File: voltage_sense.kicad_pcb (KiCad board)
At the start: 6 copper layers, 48 x 34 mm, 58 parts, among them IC1 DAC101C081CIMK_NOPB, J1 Conn_Coaxial, J2 Conn_01x04, J4 HDMI_A, J5 Conn_Coaxial, U1 OPA188xxDBV, U2 ADA4000-1, U3 OPA188xxDBV, U4 MCP4017T-103E_LT, U5 OPA1641, U6 24AA025UID, U9 LP2981A-33DBVT

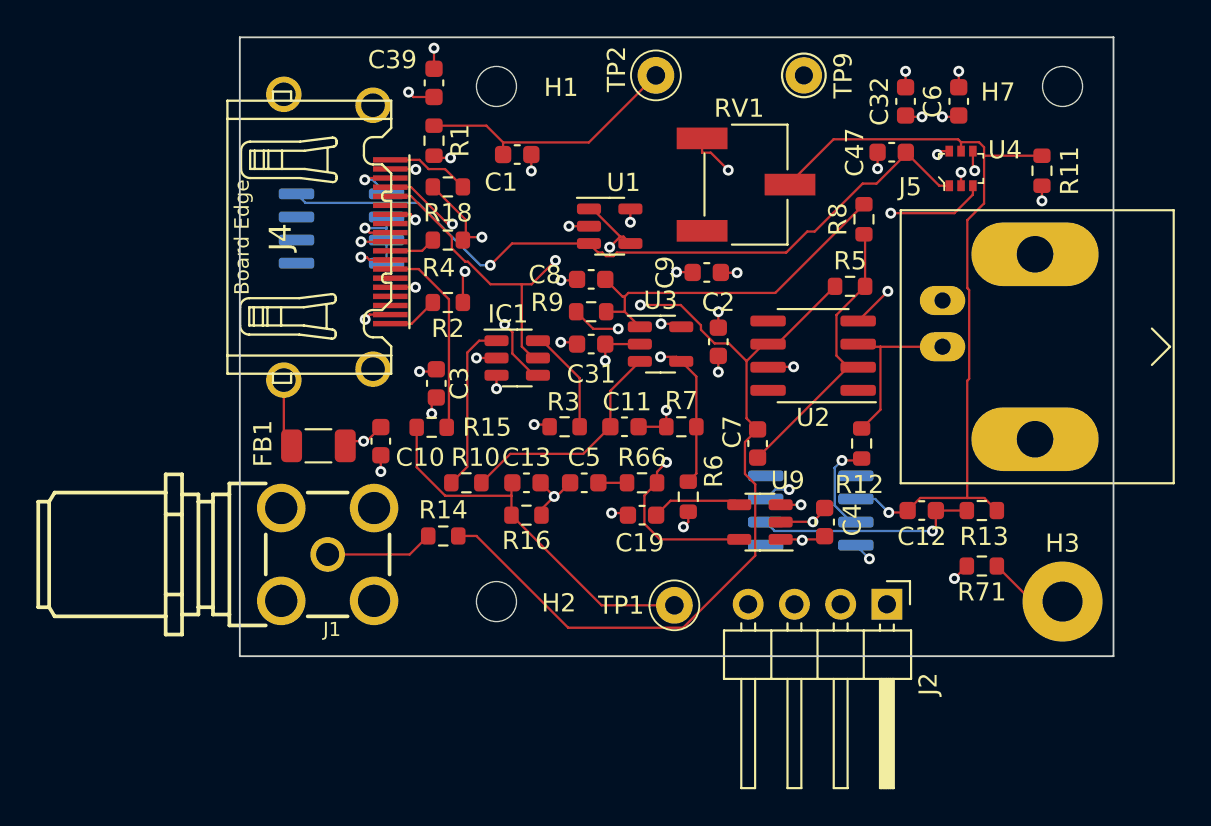
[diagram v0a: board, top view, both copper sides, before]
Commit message: Add files via upload
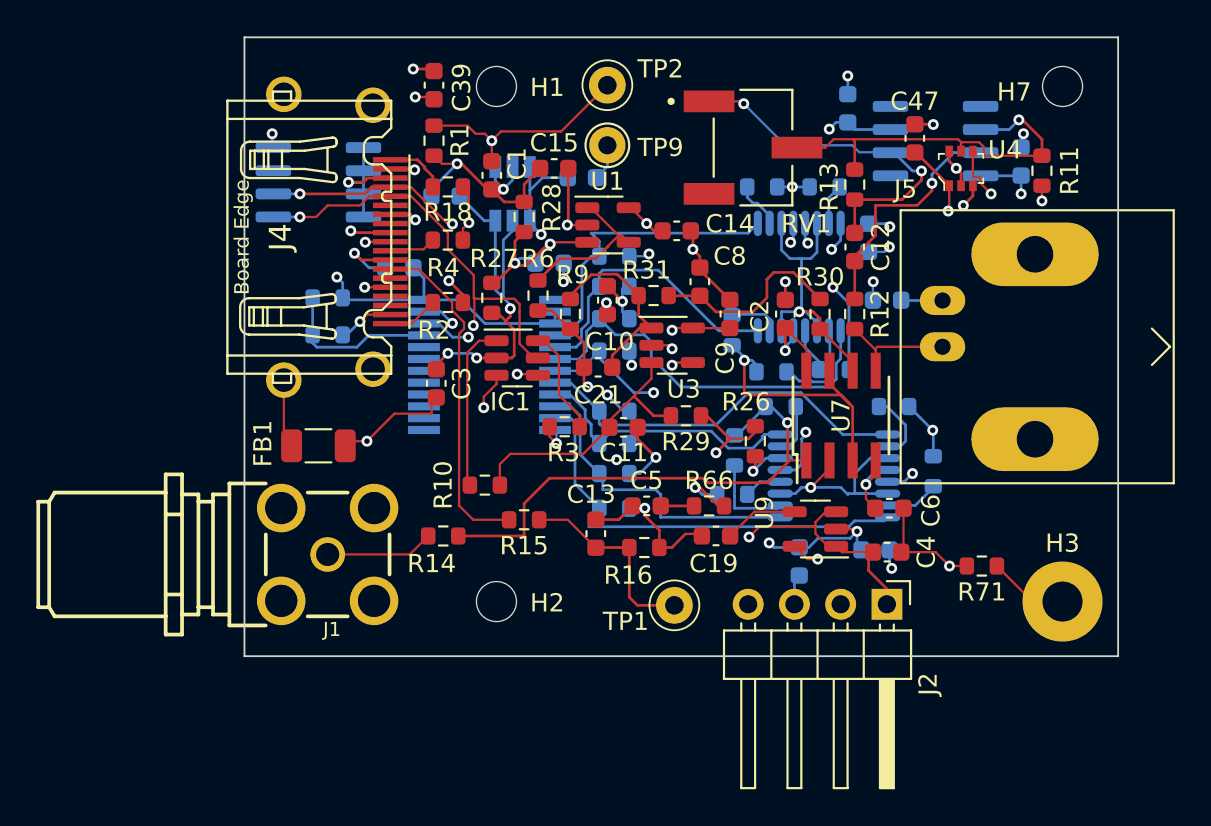
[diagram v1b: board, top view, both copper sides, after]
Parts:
- removed R7: 27.4k, Resistor_SMD:R_0603_1608Metric
- added C14: 0.1u, Capacitor_SMD:C_0603_1608Metric, F.Cu at (24.0, -23.4)
- added C15: 0.1u, Capacitor_SMD:C_0603_1608Metric, F.Cu at (17.3, -26.8)
- added C16: 0.1u, Capacitor_SMD:C_0603_1608Metric, B.Cu at (35.6, -19.6)
- added C17: 0.1u, Capacitor_SMD:C_0603_1608Metric, B.Cu at (34.5, -23.0)
- added C18: 0.1u, Capacitor_SMD:C_0603_1608Metric, B.Cu at (30.7, -5.21)
- added C20: 0.1u, Capacitor_SMD:C_0603_1608Metric, B.Cu at (34.9, -5.84)
- added C21: 10p, Capacitor_SMD:C_0603_1608Metric, F.Cu at (19.7, -15.9)
- added C22: 0.1u, Capacitor_SMD:C_0603_1608Metric, B.Cu at (18.8, -26.3)
- added C23: 1u, Capacitor_SMD:C_0603_1608Metric, B.Cu at (11.3, -25.3)
- added C24: 1u, Capacitor_SMD:C_0603_1608Metric, B.Cu at (17.0, -21.6)
- added R17: 100k, Resistor_SMD:R_0603_1608Metric, B.Cu at (20.6, -22.0)
- added R19: 100k, Resistor_SMD:R_0603_1608Metric, B.Cu at (20.6, -13.5)
- added R20: 100k, Resistor_SMD:R_0603_1608Metric, B.Cu at (20.6, -20.3)
- added R21: 100k, Resistor_SMD:R_0603_1608Metric, B.Cu at (20.6, -11.7)
- added R22: 100k, Resistor_SMD:R_0603_1608Metric, B.Cu at (20.6, -18.5)
- added R23: 100k, Resistor_SMD:R_0603_1608Metric, B.Cu at (20.6, -10.0)
- added R24: 100k, Resistor_SMD:R_0603_1608Metric, B.Cu at (20.6, -16.8)
- added R25: 100k, Resistor_SMD:R_0603_1608Metric, B.Cu at (20.6, -8.13)
- added R26: 3.01k, Resistor_SMD:R_0603_1608Metric, F.Cu at (28.3, -11.8)
- added R27: 10k, Resistor_SMD:R_0603_1608Metric, F.Cu at (13.8, -19.7)
- added R28: 10k, Resistor_SMD:R_0603_1608Metric, F.Cu at (15.6, -24.1)
- added R29: 4.99k, Resistor_SMD:R_0603_1608Metric, F.Cu at (24.5, -13.2)
- added R30: 3.01k, Resistor_SMD:R_0603_1608Metric, F.Cu at (31.9, -18.8)
- added R31: 49.9, Resistor_SMD:R_0603_1608Metric, F.Cu at (22.7, -19.8)
- added R32: DNI, Resistor_SMD:R_0603_1608Metric, B.Cu at (32.6, -15.7)
- added R33: 226k, Resistor_SMD:R_0603_1608Metric, B.Cu at (28.7, -25.8)
- added R34: 348k, Resistor_SMD:R_0603_1608Metric, B.Cu at (27.1, -17.9)
- added R35: 470k, Resistor_SMD:R_0603_1608Metric, B.Cu at (29.2, -15.6)
- added R36: 604k, Resistor_SMD:R_0603_1608Metric, B.Cu at (32.1, -25.8)
- added R38: DNI, Resistor_SMD:R_0603_1608Metric, B.Cu at (27.1, -8.89)
- added R39: 226k, Resistor_SMD:R_0603_1608Metric, B.Cu at (35.9, -13.7)
- added R40: 348k, Resistor_SMD:R_0603_1608Metric, B.Cu at (29.7, -13.7)
- added R41: 470k, Resistor_SMD:R_0603_1608Metric, B.Cu at (27.2, -11.3)
- added R42: 604k, Resistor_SMD:R_0603_1608Metric, B.Cu at (38.1, -10.2)
- added U10: TMUX6111PWR, covg-kicad:PW0016A_N, B.Cu at (32.6, -9.91)
- added U11: REF3440TIDBVR, covg-kicad:REF3440, B.Cu at (15.0, -25.4)
- added U7: ADA4000-2ARZ-R7, covg-kicad:R_8_ADI, F.Cu at (33.0, -13.2)
- added U8: TMUX6111PWR, covg-kicad:PW0016A_N, B.Cu at (30.7, -20.8)
- C11: value 0.1u -> 1u
- C31, C32: moved to B.Cu
- C7: value 4p -> 0.1u; moved to B.Cu
- C8: value 0.1u -> 1n
- J2: value Conn_01x04 -> DNI
- R10: value 27.4k -> 49.9k
- R12: value DNI -> 0
- R5: value 60.4k -> 100k; moved to B.Cu
- R6: value 33.2k -> 49.9k
- R8: value 3.01k -> DNI; moved to B.Cu
- R9: value 10k -> 4.99k
- RV1: footprint Potentiometer_SMD:Potentiometer_Bourns_3269W_Vertical -> covg-kicad:TRIM_3269W-1-103GLF
- U2: value ADA4000-1 -> TCA9555DBR; footprint Package_SO:SOIC-8_3.9x4.9mm_P1.27mm -> Package_SO:SSOP-24_5.3x8.2mm_P0.65mm; moved to B.Cu
- moved R8 30.1 mm to (4.83, -17.7), turned to 0 degrees
- moved R5 28.7 mm to (4.83, -19.7)
- moved C31 25.7 mm to (42.9, -27.2), turned to -90 degrees
- moved C6 22.7 mm to (35.7, -8.13), turned to 0 degrees
- moved C7 21.9 mm to (8.76, -21.3), turned to 0 degrees
- moved U5 21.4 mm to (38.2, -28.3)
- moved R13 19.2 mm to (33.8, -25.9), turned to 90 degrees
- moved U2 17.8 mm to (13.7, -16.0)
- moved C12 14.9 mm to (33.8, -22.5), turned to -90 degrees
- moved C10 14.7 mm to (20.2, -19.6)
- moved R6 13.8 mm to (16.4, -19.8), turned to 90 degrees
- moved TP9 11.5 mm to (20.2, -28.1)
- moved R15 7.18 mm to (15.6, -7.49), turned to 180 degrees
- moved R12 7.12 mm to (33.8, -18.8), turned to -90 degrees
- moved R16 6.72 mm to (22.2, -5.97)
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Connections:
- net 3V3_BUF renamed /vsense/2V_BUF
- C3 pad 2: +5V -> +4V
- C7 pad 1: Net-(C7-Pad1) -> GND
- C7 pad 2: Net-(C7-Pad2) -> +3V3
- IC1 pad 2: +5V -> +4V
- IC1 pad 4: /vsense/SDA -> SDA
- IC1 pad 5: /vsense/SCL -> SCL
- J4 pad 15: /vsense/SCL -> SCL
- J4 pad 16: /vsense/SDA -> SDA
- R11 pad 2: Net-(C12-Pad2) -> Net-(R11-Pad2)
- R12 pad 1: Net-(R12-Pad1) -> Net-(C12-Pad2)
- R13 pad 2: Net-(C12-Pad2) -> Net-(R11-Pad2)
- R14 pad 2: Net-(C7-Pad2) -> /vsense/gain_adjust_2/OUT
- R18 pad 1: /vsense/AMP_OUT -> /vsense/STG1_OUT
- R18 pad 2: Net-(C7-Pad2) -> /vsense/AMP_OUT
- R4 pad 1: /vsense/CAL_ADC -> /vsense/STG1_OUT
- R4 pad 2: Net-(C7-Pad2) -> /vsense/CAL_ADC
- R5 pad 1: Net-(C7-Pad1) -> +3V3
- R5 pad 2: Net-(C7-Pad2) -> Net-(R5-Pad2)
- R8 pad 1: Net-(C7-Pad1) -> Net-(R5-Pad2)
- R8 pad 2: Net-(C8-Pad2) -> GND
- R9 pad 1: Net-(C8-Pad2) -> /vsense/OFF_ADJ
- RV1 pad 2: Net-(C12-Pad2) -> Net-(R11-Pad2)
- U1 pad 3: +3V3 -> Net-(C24-Pad2)
- U2 pad 2: Net-(C7-Pad1) -> +3V3
- U2 pad 3: Net-(J5-Pad1) -> +3V3
- U2 pad 4: -15V -> /vsense/SW0
- U2 pad 5: unconnected-(U2-Pad5) -> /vsense/SW1
- U2 pad 6: Net-(C7-Pad2) -> /vsense/SW2
- U2 pad 7: +15V -> /vsense/SW3
- U2 pad 8: unconnected-(U2-Pad8) -> /vsense/SW4
- U3 pad 1: Net-(C8-Pad2) -> /vsense/OFF_ADJ
- U4 pad 3: /vsense/SCL -> SCL
- U4 pad 4: /vsense/SDA -> SDA
- U4 pad 5: Net-(C12-Pad2) -> Net-(R11-Pad2)
- U5 pad 2: Net-(C12-Pad2) -> Net-(R11-Pad2)
- U5 pad 3: Net-(R12-Pad1) -> Net-(C12-Pad2)
- U6 pad 5: /SDA -> SCL
- U6 pad 6: /SCL -> SDA
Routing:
- net GND: track 40.5 -> 105.0 mm, vias 27 -> 32
- net Net-(C7-Pad2): track 60.2 -> 0.00 mm, vias 2 -> 0
- net SDA: track 0.00 -> 59.2 mm, vias 0 -> 5
- net SCL: track 0.00 -> 57.7 mm, vias 0 -> 4
- net +5V: track 8.02 -> 57.9 mm, vias 6 -> 5
- net /vsense/STG1_OUT: track 0.00 -> 46.5 mm, vias 0 -> 3
- net /vsense/SDA: track 45.1 -> 0.00 mm, vias 3 -> 0
- net /vsense/SCL: track 41.5 -> 0.00 mm, vias 2 -> 0
- net /vsense/gain_adjust_2/OUT: track 0.00 -> 39.7 mm, vias 0 -> 2
- net +3V3: track 65.7 -> 30.8 mm, vias 2 -> 6
- net Net-(C12-Pad2): track 44.0 -> 13.1 mm
- net /vsense/SW7: track 0.00 -> 24.3 mm
- net /vsense/SW2: track 0.00 -> 22.0 mm
- net /vsense/SW3: track 0.00 -> 21.9 mm, vias 0 -> 2
- net Net-(R11-Pad2): track 0.00 -> 21.4 mm, vias 0 -> 1
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- added copper zone on In2.Cu, net +3V3
- removed copper zone on In2.Cu, net +5V

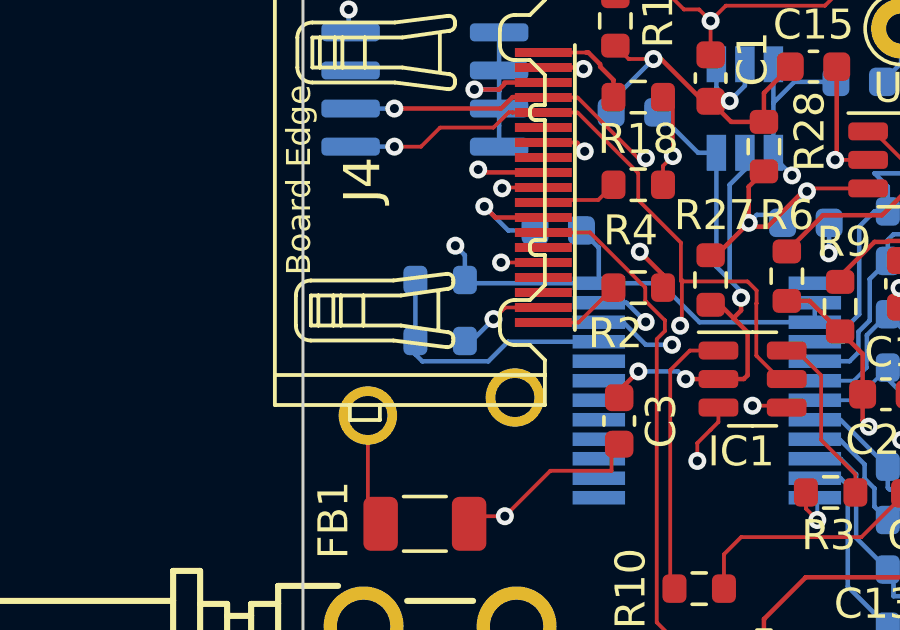
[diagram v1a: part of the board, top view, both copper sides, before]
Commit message: All production files in jlcpcb/production_files
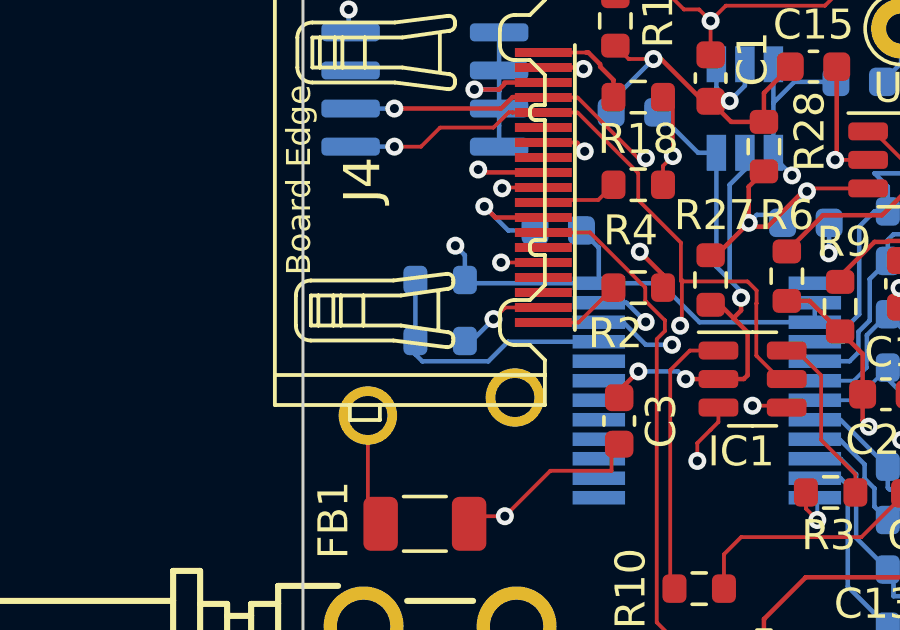
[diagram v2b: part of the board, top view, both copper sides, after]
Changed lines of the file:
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@@
     (descr "http://www.farnell.com/datasheets/612848.pdf")
     (tags "BNC Amphenol Horizontal")
-    (property "Manf#" "C2874827")
     (property "Sheetfile" "voltage_sense_top.kicad_sch")
     (property "Sheetname" "vsense")
@@
     (fp_arc (start 5.5 -3) (mid 5.353553 -2.646447) (end 5 -2.5) (layer "F.SilkS") (width 0.127))
     (fp_arc (start 4.5 -2.5) (mid 4.146447 -2.646447) (end 4 -3) (layer "F.SilkS") (width 0.127))
-    (fp_arc (start 5.075468 -0.778281) (mid 5.142434 -0.901086) (end 5.273459 -0.949998) (layer "F.SilkS") (width 0.127))
+    (fp_arc (start 5.075468 -0.778281) (mid 5.142414 -0.901105) (end 5.273459 -0.949998) (layer "F.SilkS") (width 0.127))
     (fp_arc (start -5.4719 -0.7752) (mid -5.423377 -0.932365) (end -5.273441 -1.000001) (layer "F.SilkS") (width 0.127))
     (fp_arc (start -3.25 3.75) (mid -3.396447 4.103553) (end -3.75 4.25) (layer "F.SilkS") (width 0.127))
     (fp_arc (start -5 -2.5) (mid -5.353553 -2.646447) (end -5.5 -3) (layer "F.SilkS") (width 0.127))
     (fp_arc (start -2 -3.7) (mid -2.058579 -3.558579) (end -2.2 -3.5) (layer "F.SilkS") (width 0.127))
-    (fp_arc (start 5.373443 -0.95) (mid 5.523389 -0.882352) (end 5.571899 -0.725198) (layer "F.SilkS") (width 0.127))
+    (fp_arc (start 5.373443 -0.95) (mid 5.523346 -0.882348) (end 5.571899 -0.725198) (layer "F.SilkS") (width 0.127))
     (fp_arc (start 2.2 -3.5) (mid 2.058579 -3.558579) (end 2 -3.7) (layer "F.SilkS") (width 0.127))
-    (fp_arc (start 3.42654 -0.95) (mid 3.557588 -0.901082) (end 3.62453 -0.778279) (layer "F.SilkS") (width 0.127))
+    (fp_arc (start 3.42654 -0.95) (mid 3.55756 -0.901074) (end 3.62453 -0.778279) (layer "F.SilkS") (width 0.127))
     (fp_arc (start 5.35 3.8) (mid 5.203553 4.153553) (end 4.85 4.3) (layer "F.SilkS") (width 0.127))
     (fp_arc (start -2.3 -3.5) (mid -2.441421 -3.558579) (end -2.5 -3.7) (layer "F.SilkS") (width 0.127))
@@
     (fp_line (start -1.113417 1.125451) (end -1.081286 1.125451) (layer "B.Fab") (width 0.127))
     (fp_line (start 1.421808 0.750547) (end 1.421808 1.125451) (layer "B.Fab") (width 0.127))
-    (fp_arc (start -0.576537 0.906071) (mid -0.449563 0.779101) (end -0.322588 0.906071) (layer "B.Fab") (width 0.127))
+    (fp_arc (start -0.576537 0.906071) (mid -0.449563 0.779106) (end -0.322588 0.906071) (layer "B.Fab") (width 0.127))
     (fp_arc (start -0.724999 1.446) (mid -0.778512 1.423533) (end -0.800692 1.369901) (layer "B.Fab") (width 0.127))
     (fp_arc (start -0.800692 -1.398928) (mid -0.778507 -1.452548) (end -0.724999 -1.475002) (layer "B.Fab") (width 0.127))
@@
     (connect_pads (clearance 0))
     (min_thickness 0.254)
-    (keepout (tracks allowed) (vias allowed) (pads allowed) (copperpour not_allowed) (footprints allowed))
+    (keepout (tracks allowed) (vias allowed) (pads allowed ) (copperpour not_allowed) (footprints allowed))
     (fill (thermal_gap 0.508) (thermal_bridge_width 0.508))
     (polygon
@@
     (connect_pads (clearance 0))
     (min_thickness 0.254)
-    (keepout (tracks allowed) (vias allowed) (pads allowed) (copperpour not_allowed) (footprints allowed))
+    (keepout (tracks allowed) (vias allowed) (pads allowed ) (copperpour not_allowed) (footprints allowed))
     (fill (thermal_gap 0.508) (thermal_bridge_width 0.508))
     (polygon
